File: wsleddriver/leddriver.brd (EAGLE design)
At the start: 35.2 x 13.7 mm, 15 parts, among them IC1 WS2811-SOP8

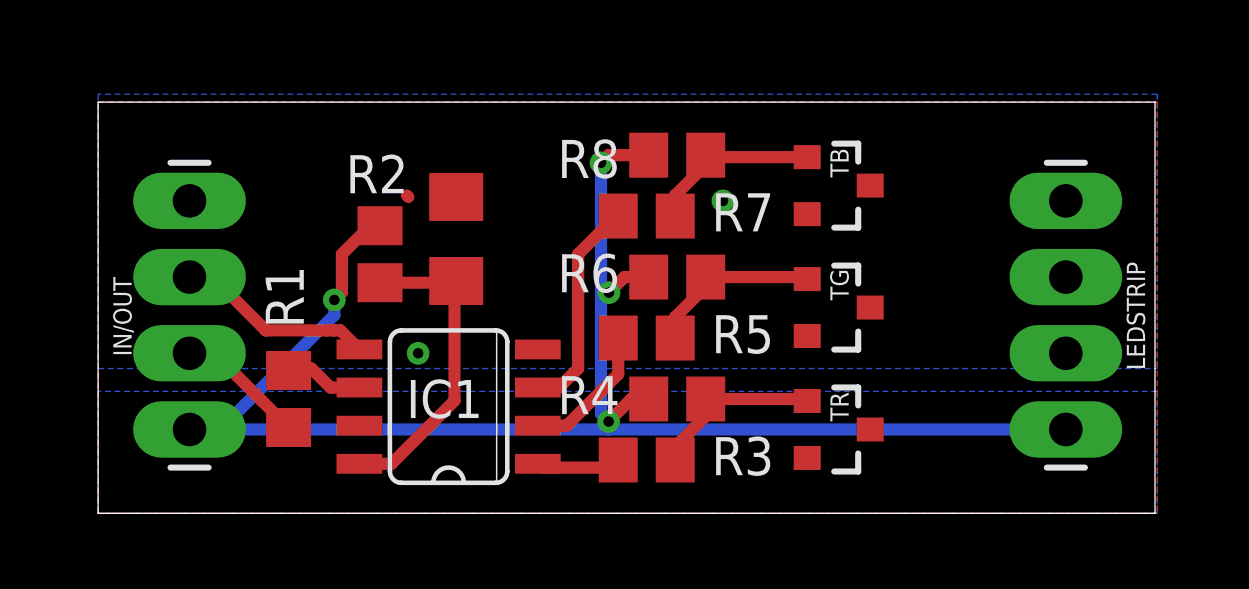
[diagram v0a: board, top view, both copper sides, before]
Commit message: a
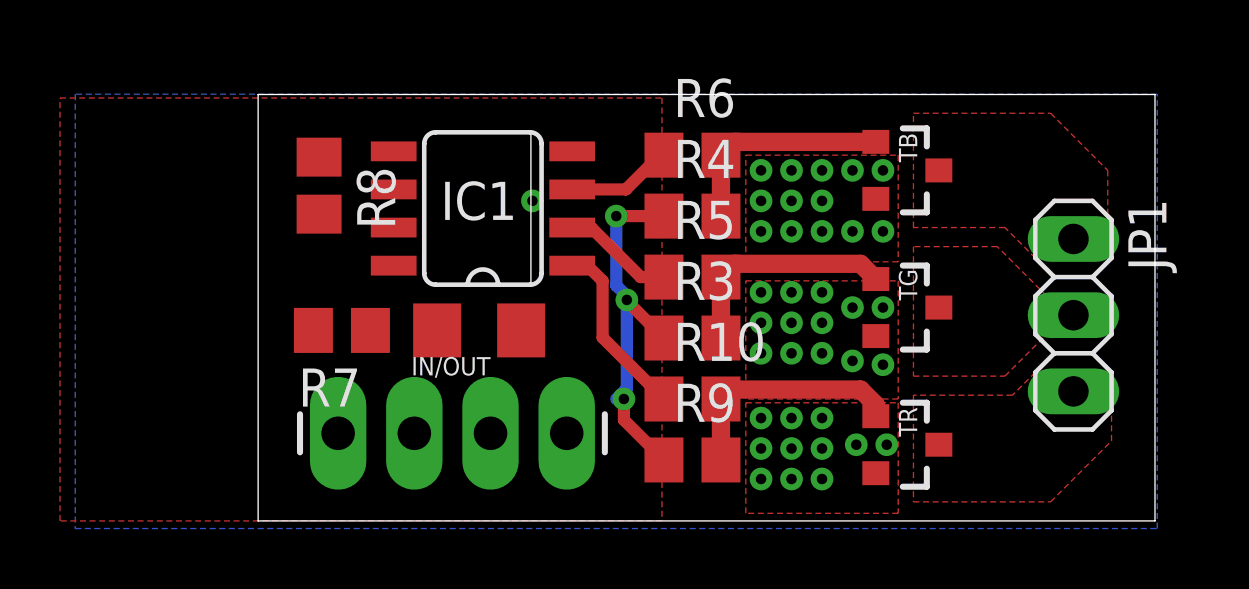
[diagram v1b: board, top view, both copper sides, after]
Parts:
- removed LEDSTRIP: (no value), SparkFun-Connectors:1X04_LONGPADS
- removed R1: 33, rcl:R0805
- removed R2: 2.7K, rcl:R0805
- added JP1: (no value), pinhead:1X03
- added R10: 100, rcl:R0805
- added R9: 10k, rcl:R0805
- R3: value 100 -> 10k
- R4: value 10K -> 10k
- R6: value 10K -> 100
- R7: value 100 -> 2.7k
- R8: value 10K -> 33
- moved IN/OUT 14.8 mm to (15.6, 2.67), turned to 180 degrees
- moved R8 12.0 mm to (7.37, 10.9), turned to 270 degrees
- moved R7 10.9 mm to (8.13, 6.10), turned to 180 degrees
- moved IC1 6.70 mm to (12.8, 10.2)
- moved R4 6.12 mm to (19.8, 9.91)
- moved R3 4.34 mm to (19.8, 5.84)
- moved R6 4.10 mm to (19.8, 11.9)
- moved C1 3.14 mm to (12.7, 6.10), turned to 180 degrees
- moved R5 2.54 mm to (19.8, 7.87)
- moved TB 2.34 mm to (26.9, 11.4)
- moved TR 2.34 mm to (26.9, 2.29)
- moved TG 2.29 mm to (26.9, 6.86)
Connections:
- removed net N$5: R3.2, R4.2, TR.1
- new net N$4: R10.2, R9.2, TR.1
- net +12V: now also R3.1, R7.2, R9.1; no longer LEDSTRIP.4, R2.2, R6.1, R8.1
- net B: now also R6.1; no longer R7.1
- net DIN_IN: now also R8.2; no longer R1.2
- net N$1: now also R8.1; no longer R1.1
- net N$2: now also R3.2; no longer R6.2
- net N$3: now also R4.2, R6.2; no longer R7.2, R8.2
- net NEG_B: now also JP1.1; no longer LEDSTRIP.1
- net NEG_G: now also JP1.2; no longer LEDSTRIP.2
- net NEG_R: now also JP1.3; no longer LEDSTRIP.3
- net R: now also R10.1; no longer R3.1
- net VDD: now also R7.1; no longer R2.1
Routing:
- net +12V: track 53.5 -> 12.3 mm, vias 4 -> 3
- net VDD: track 10.5 -> 0.00 mm
- net N$4: track 0.00 -> 8.25 mm
- net DOUT_OUT: track 6.66 -> 0.51 mm
- net N$5: track 5.86 -> 0.00 mm
- net DIN_IN: track 4.33 -> 0.00 mm
- net B: track 7.28 -> 3.54 mm
- net R: track 2.84 -> 6.01 mm
- net N$1: track 2.65 -> 0.52 mm
- net N$2: track 5.86 -> 7.92 mm
- net N$3: track 6.57 -> 7.38 mm
- net GND: track 0.32 -> 0.00 mm, vias 2 -> 38
- added copper zone on layer 1, net NEG_B
- added copper zone on layer 1, net NEG_G
- added copper zone on layer 1, net NEG_R
- removed copper zone on layer 16, net +12V
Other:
- board size 35.2 x 13.7 mm -> 29.9 x 14.2 mm
